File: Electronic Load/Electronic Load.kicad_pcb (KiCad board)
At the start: 2 copper layers, 27 parts, among them J1 Load_IN, J2 Fan Connector, J3 Programming Header, J4 Load_OUT, J5 USB_C_Receptacle, Q1 IRFS3306, Q2 IRFS3306, Q3 IRFS3306, Q4 IRFS3306, SW1 Rotary_Encoder_Switch, U1 ATtiny84-20SSU, U2 MCP4551, U3 SSD1306, U4 OPA2277, U5 ACS758xCB-150U-PFF

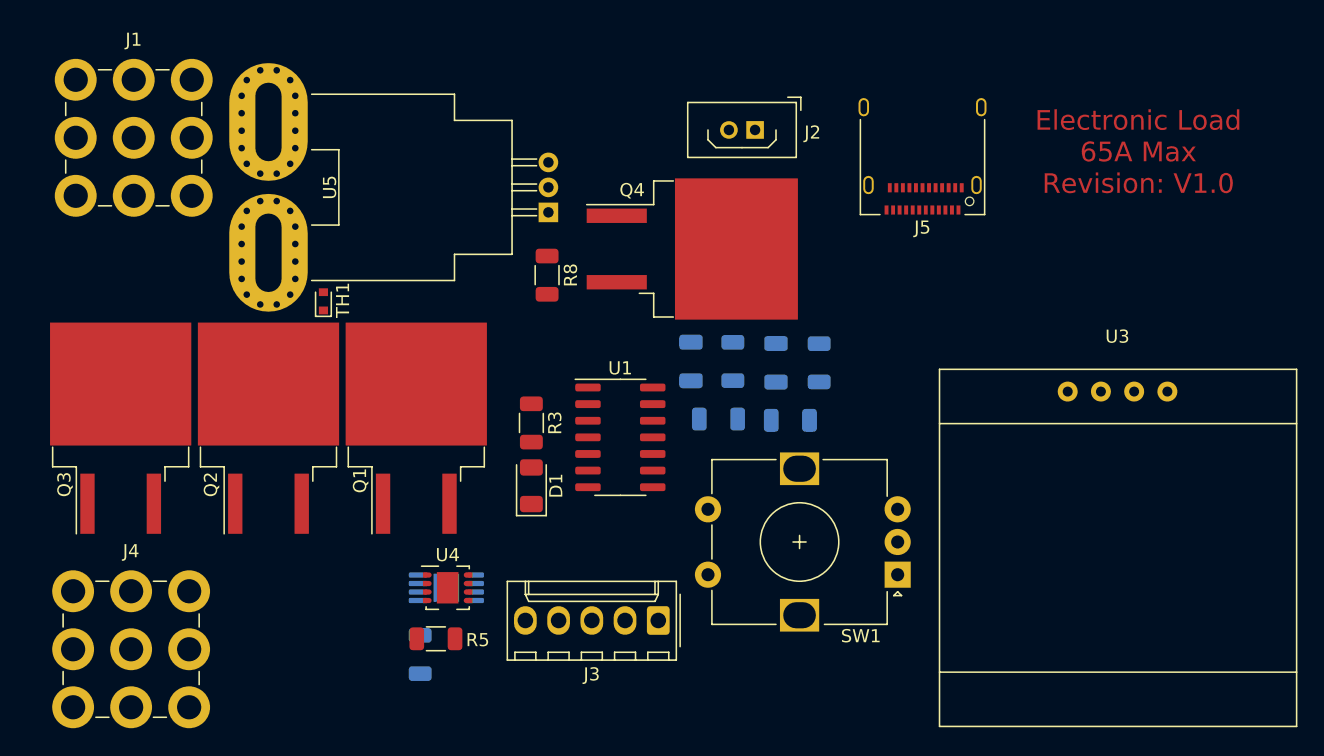
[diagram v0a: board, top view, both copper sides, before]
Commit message: Updated PCB
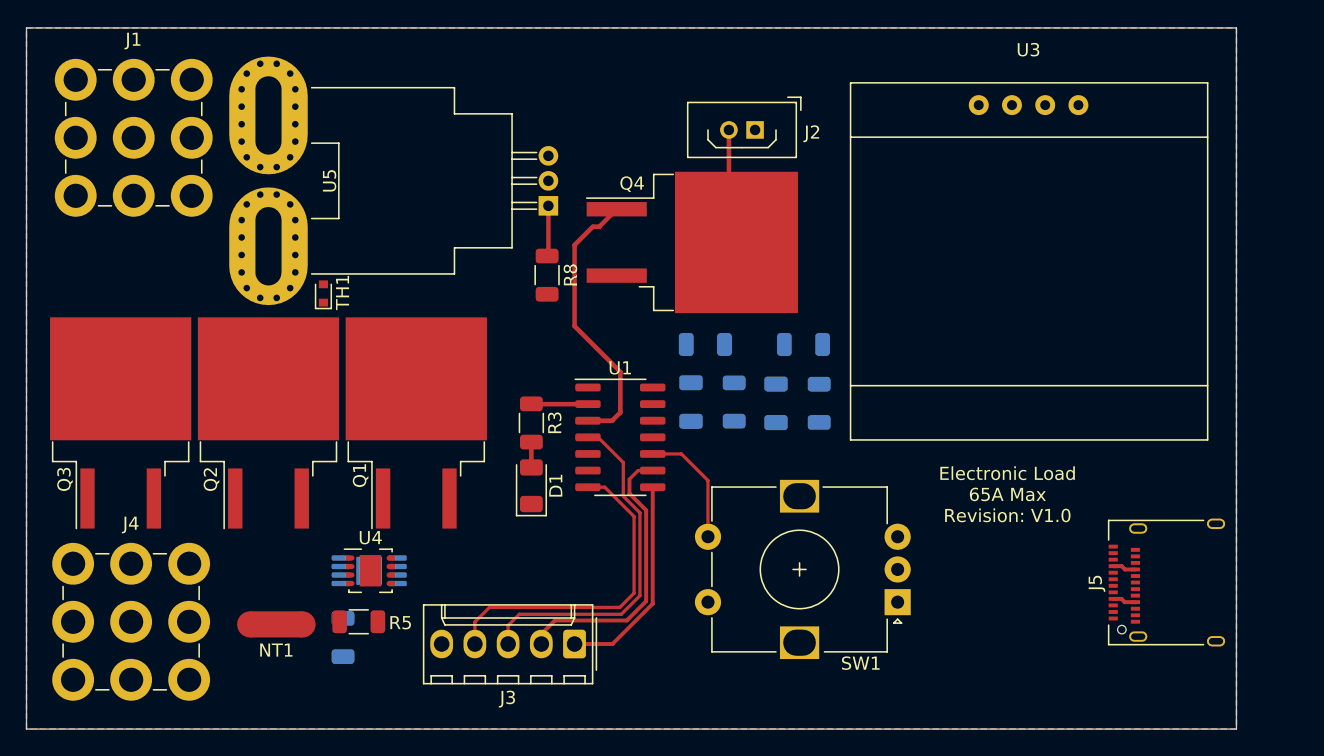
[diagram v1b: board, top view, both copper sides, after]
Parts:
- added NT1: Net-Tie_2, NetTie:NetTie-2_SMD_Pad2.0mm, F.Cu at (105.0, 88.3)
- moved J5 38.8 mm to (174.0, 85.1), turned to 90 degrees
- moved U3 22.9 mm to (148.9, 46.9)
- moved J3 6.65 mm to (127.8, 89.8)
- moved R5 6.04 mm to (111.3, 88.1)
- moved R4 6.04 mm to (110.1, 89.3)
- moved U2 6.04 mm to (112.1, 84.2)
- moved U4 6.04 mm to (112.2, 84.2)
- moved C2 3.10 mm to (143.2, 71.4)
- moved C1 3.10 mm to (136.7, 71.3)
- moved R6 2.56 mm to (146.5, 71.4), turned to 270 degrees
- moved R1 2.47 mm to (137.8, 66.9), turned to 0 degrees
- moved J4 2.10 mm to (93.9, 88.1)
- moved SW1 2.10 mm to (152.5, 86.6)
- moved R2 1.84 mm to (145.3, 66.9), turned to 0 degrees
- moved R7 1.77 mm to (140.0, 71.3), turned to 90 degrees
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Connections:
- C1 pad 2: RETURN -> GND
- C2 pad 1: RETURN -> GND
- D1 pad 1: RETURN -> GND
- J3 pad 1: SCL -> MISO
- J3 pad 2: MISO -> SCL
- J3 pad 3: SDA_MOSI -> RESET
- J3 pad 4: RESET -> SDA_MOSI
- J3 pad 5: RETURN -> GND
- J5 pad A1: RETURN -> GND
- J5 pad A12: RETURN -> GND
- J5 pad B1: RETURN -> GND
- J5 pad B12: RETURN -> GND
- J5 pad S1: RETURN -> GND
- Q4 pad 3: RETURN -> GND
- R5 pad 2: RETURN -> GND
- SW1 pad C: RETURN -> GND
- SW1 pad S1: RETURN -> GND
- TH1 pad 2: RETURN -> GND
- U1 pad 14: RETURN -> GND
- U1 pad 3: Net-(U1-Pad3) -> Fan_Pin
- U1 pad 5: Fan_Pin -> Net-(U1-Pad5)
- U2 pad 4: RETURN -> GND
- U3 pad 2: RETURN -> GND
- U4 pad 4: RETURN -> GND
- U5 pad 2: RETURN -> GND
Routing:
- net RESET: track 0.00 -> 26.6 mm
- net SDA_MOSI: track 0.00 -> 25.1 mm
- net SCL: track 0.00 -> 21.7 mm
- net Fan_Pin: track 0.00 -> 21.3 mm
- net MISO: track 0.00 -> 16.2 mm
- net Enc_SW: track 0.00 -> 9.37 mm
- net Net-(J2-Pad2): track 0.00 -> 8.84 mm
- net +5V: track 0.00 -> 7.49 mm
- net Net-(R3-Pad1): track 0.00 -> 4.33 mm
- net Net-(D1-Pad2): track 0.00 -> 1.94 mm
- added copper zone on B.Cu, net GND
- added copper zone on F.Cu, net GND
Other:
- board outline added: 92.5 x 53.6 mm
